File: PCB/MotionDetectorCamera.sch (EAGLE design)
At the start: 184 parts, among them J1 JUMPER-SOLDER, J12 JUMPER-AMPHENOL-10129380-9020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, J13 JUMPER-AMPHENOL-10129380-9020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, J14 JUMPER-AMPHENOL-10129380-9020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, J15 JUMPER-AMPHENOL-10129380-9020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, J2 JUMPER-SOLDER, J4 JUMPER-AMPHENOL-10129380-9020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, J5 JUMPER-SOLDER, J6 S-MOUNT-LENS-HOLDER, J7 MICROSD-SOCKET, J8 MINI-USB-JACK, Q10 PMOS-NEXPERIA-SOT1220, Q2 PMOS-NEXPERIA-SOT1220, Q3 PMOS-NEXPERIA-SOT1220, U1 NEXPERIA-74LVC1G98-BUFFER, U10 TI-TPS22919DCK, U11 TI-TPS2116, U12 TI-MSP430FR2422IRHL, U14 PANASONIC-EKMB110711X, U15 LATTICE-ICE40HX4K-BG121, U16 MICROCHIP-MCP7383X, U17 ON-AR0330CS1C12SPKA0, U18 ALLIANCE-AS4C8M16MSA-6BIN, U19 STM-STM32F730, U2 DIODESINC-AP7350, U20 DIODESINC-DT1446-04V-7, U21 NXP-NTB0102, U22 NXP-NTB0102, U23 TI-TPS6280XYKAR, U24 NEXPERIA-74LVC1G98-OR-INV-INP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, U28 NEXPERIA-74LVC1G98-NOR, U3 TI-TPS6280XYKAR, U30 TI-TPS22919DCK, U4 TI-TPS6280XYKAR, U5 WINBOND-W25Q40EW, U6 TI-TPS22919DCK, U7 TI-TPS22919DCK, U8 TI-TPS22919DCK, U9 TI-TPS22919DCK, X1 EPSON-FC-135, X2 SITIME-SIT8021, X3 SITIME-SIT8021

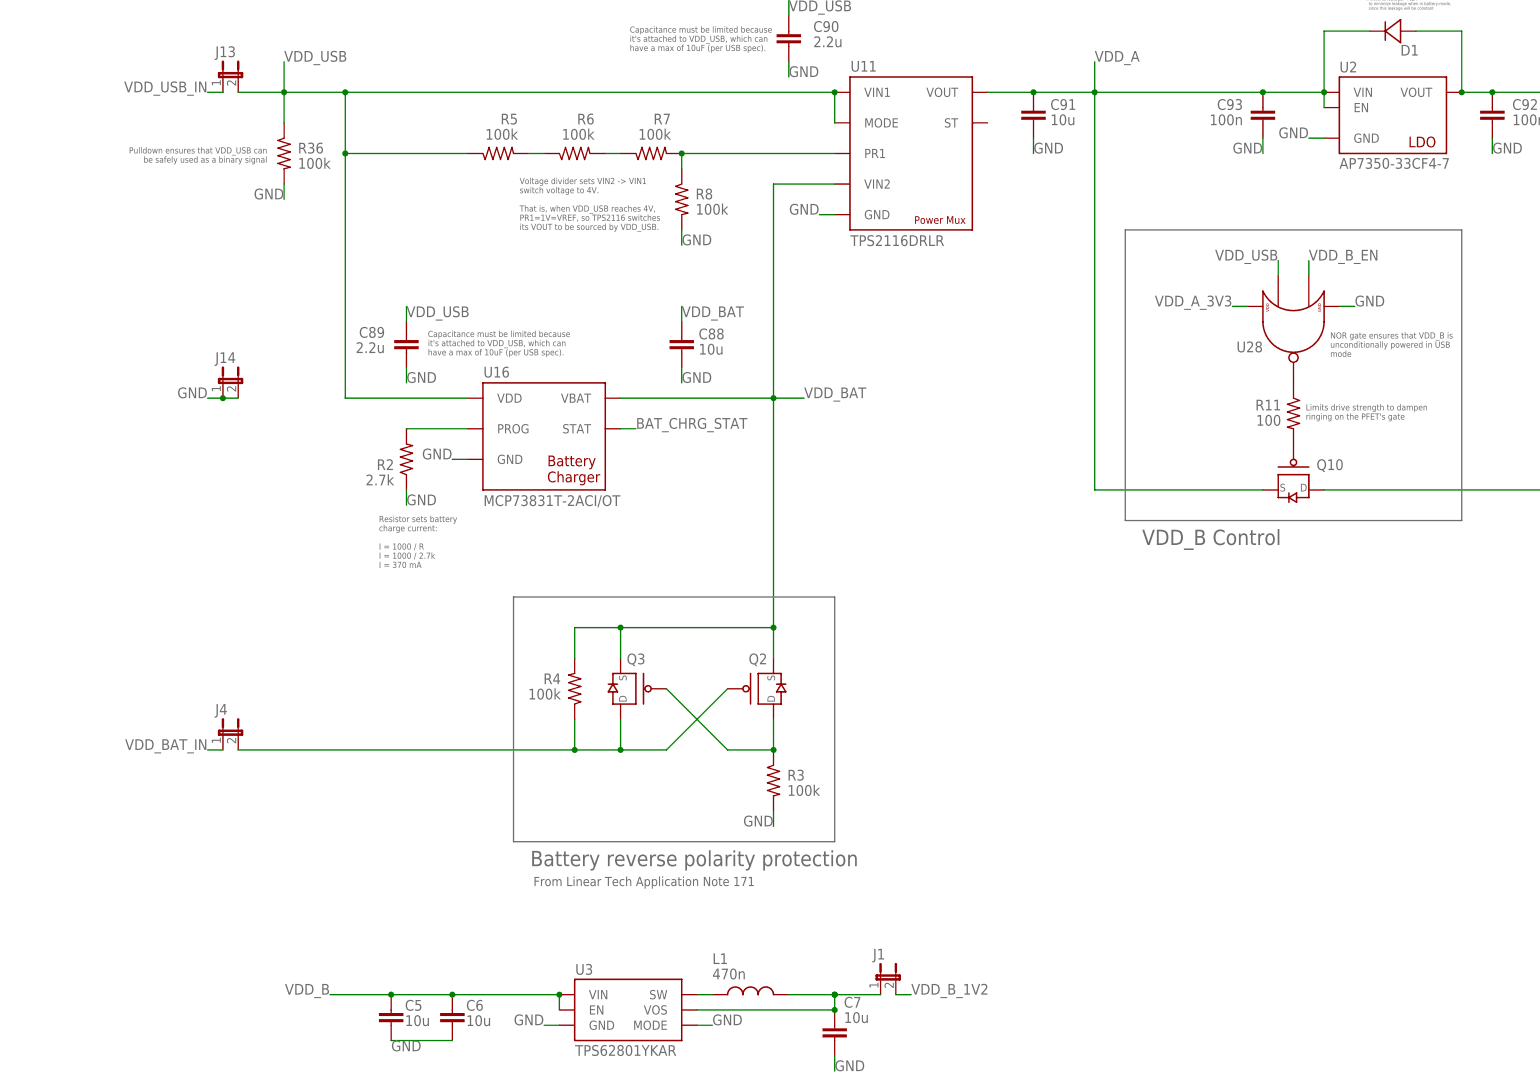
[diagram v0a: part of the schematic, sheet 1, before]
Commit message: Progress
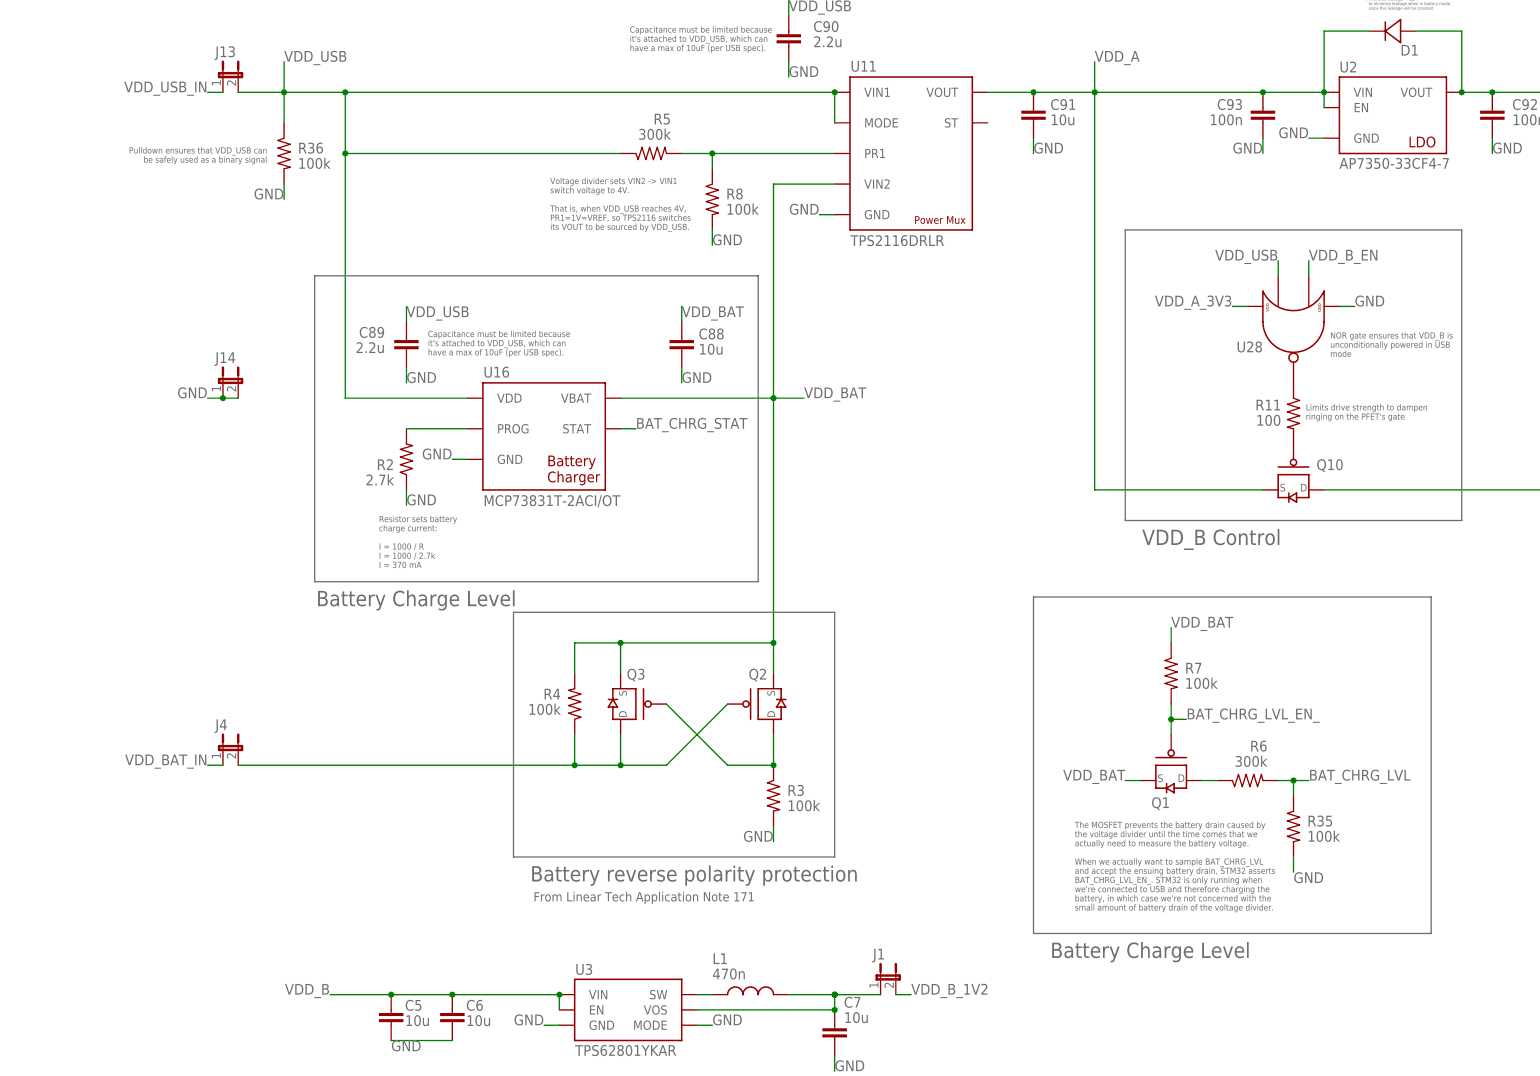
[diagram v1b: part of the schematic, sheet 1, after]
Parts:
- added Q1: PMOS-NEXPERIA-SOT1220, EagleLibrary:PMOS-NEXPERIA-SOT1220
- added R35: 100k, EagleLibrary:RESISTOR0402
- R5, R6: value 100k -> 300k; MFG Stackpole -> (none); PN RMCF0402JT100K -> (none)
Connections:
- removed net N$36: R5.2, R6.1
- removed net N$39: R6.2, R7.1
- new net BAT_CHRG_LVL: R35.1, R6.2
- new net BAT_CHRG_LVL_EN_: Q1.G, R7.2
- new net N$46: Q1.D, R6.1
- net GND: now also R35.2
- net N$42: now also R5.2; no longer R7.2
- net VDD_BAT: now also Q1.S, R7.1
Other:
- note added: "Battery Charge Level"
- note added: "The MOSFET prevents the battery drain caused by the voltage divider until the time comes that we actually need to measure the battery voltage. When we actually want to sample BAT_CHRG_LVL and accept the ensuing battery drain, STM32 asserts BAT_CHRG_LVL_EN_. STM32 is only running when we're connected to USB and therefore charging the battery, in which case we're not concerned with the small amount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"
- moved on the sheet: J4, Q2, Q3, R3, R4, R5, R6, R7, R8
